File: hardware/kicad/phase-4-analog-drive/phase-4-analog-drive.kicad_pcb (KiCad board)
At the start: 2 copper layers, 170 x 120 mm, 4 parts, among them J1 MONITOR_DRIVE, J2 HOST_CTRL, U1 SN74LV4066APWR, U2 SN74LVC1G66DBVR

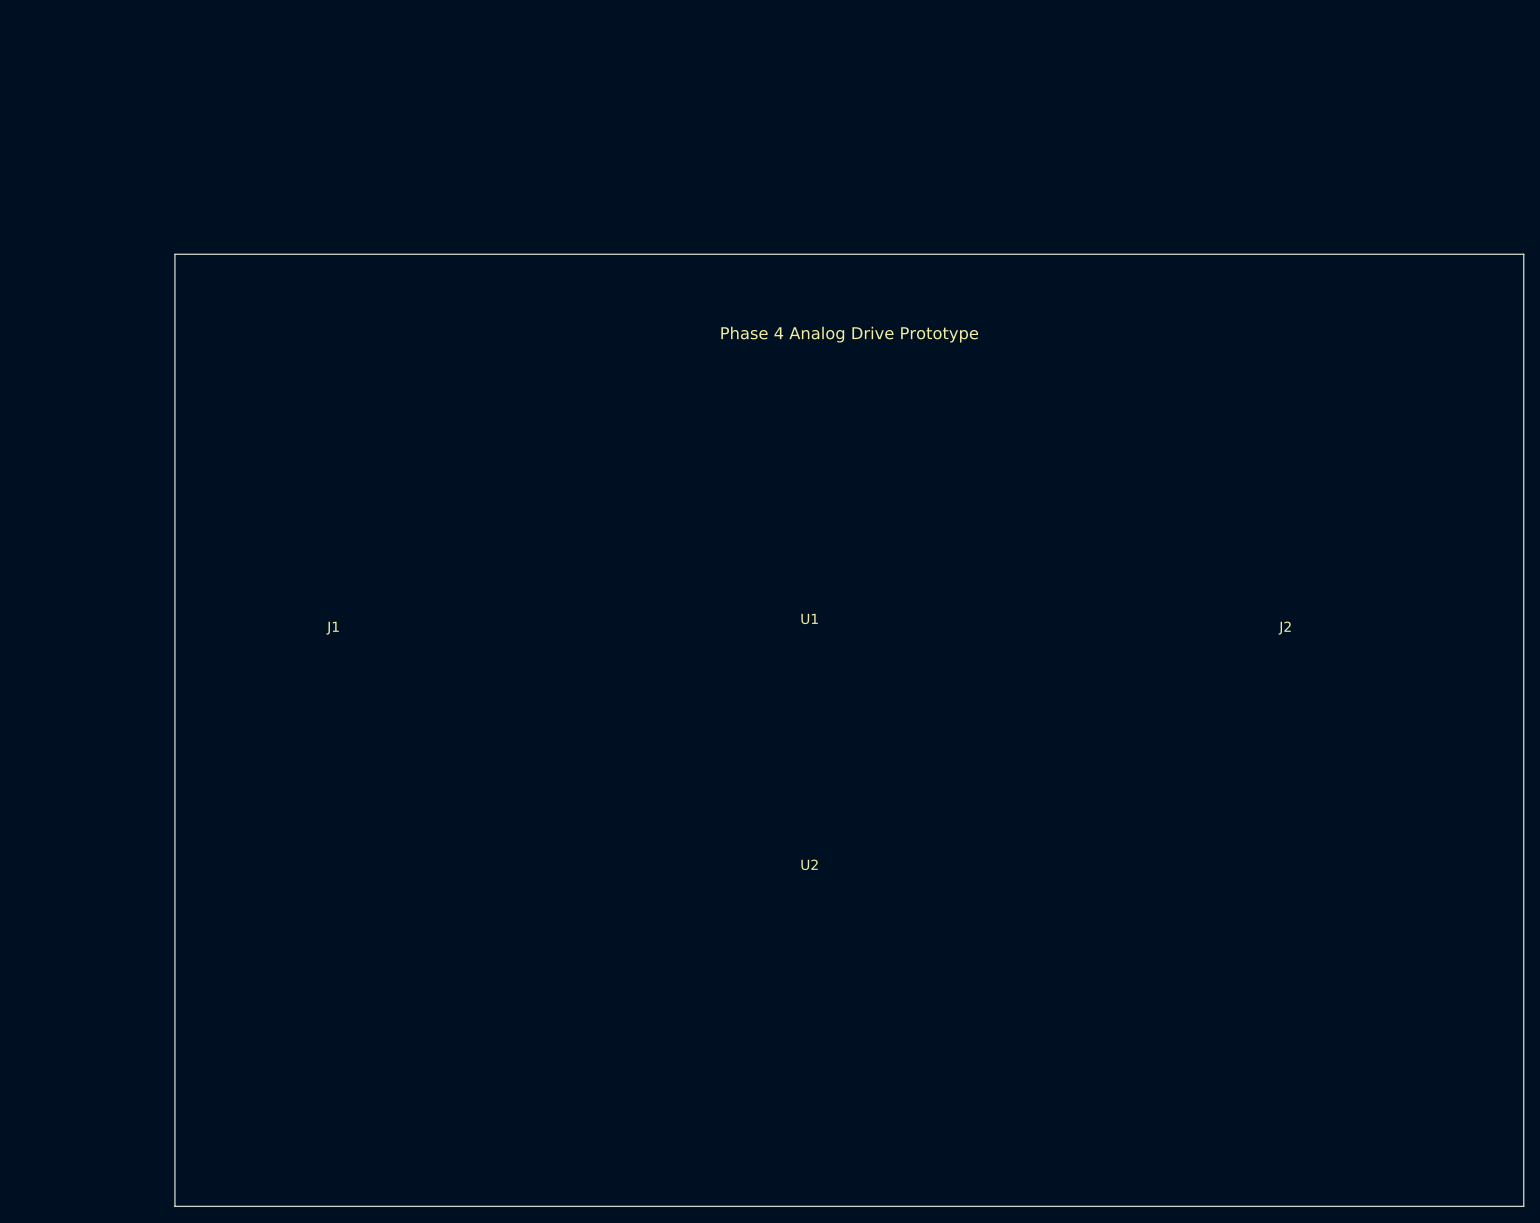
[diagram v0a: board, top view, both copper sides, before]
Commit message: Update phase 4 schema, WIP
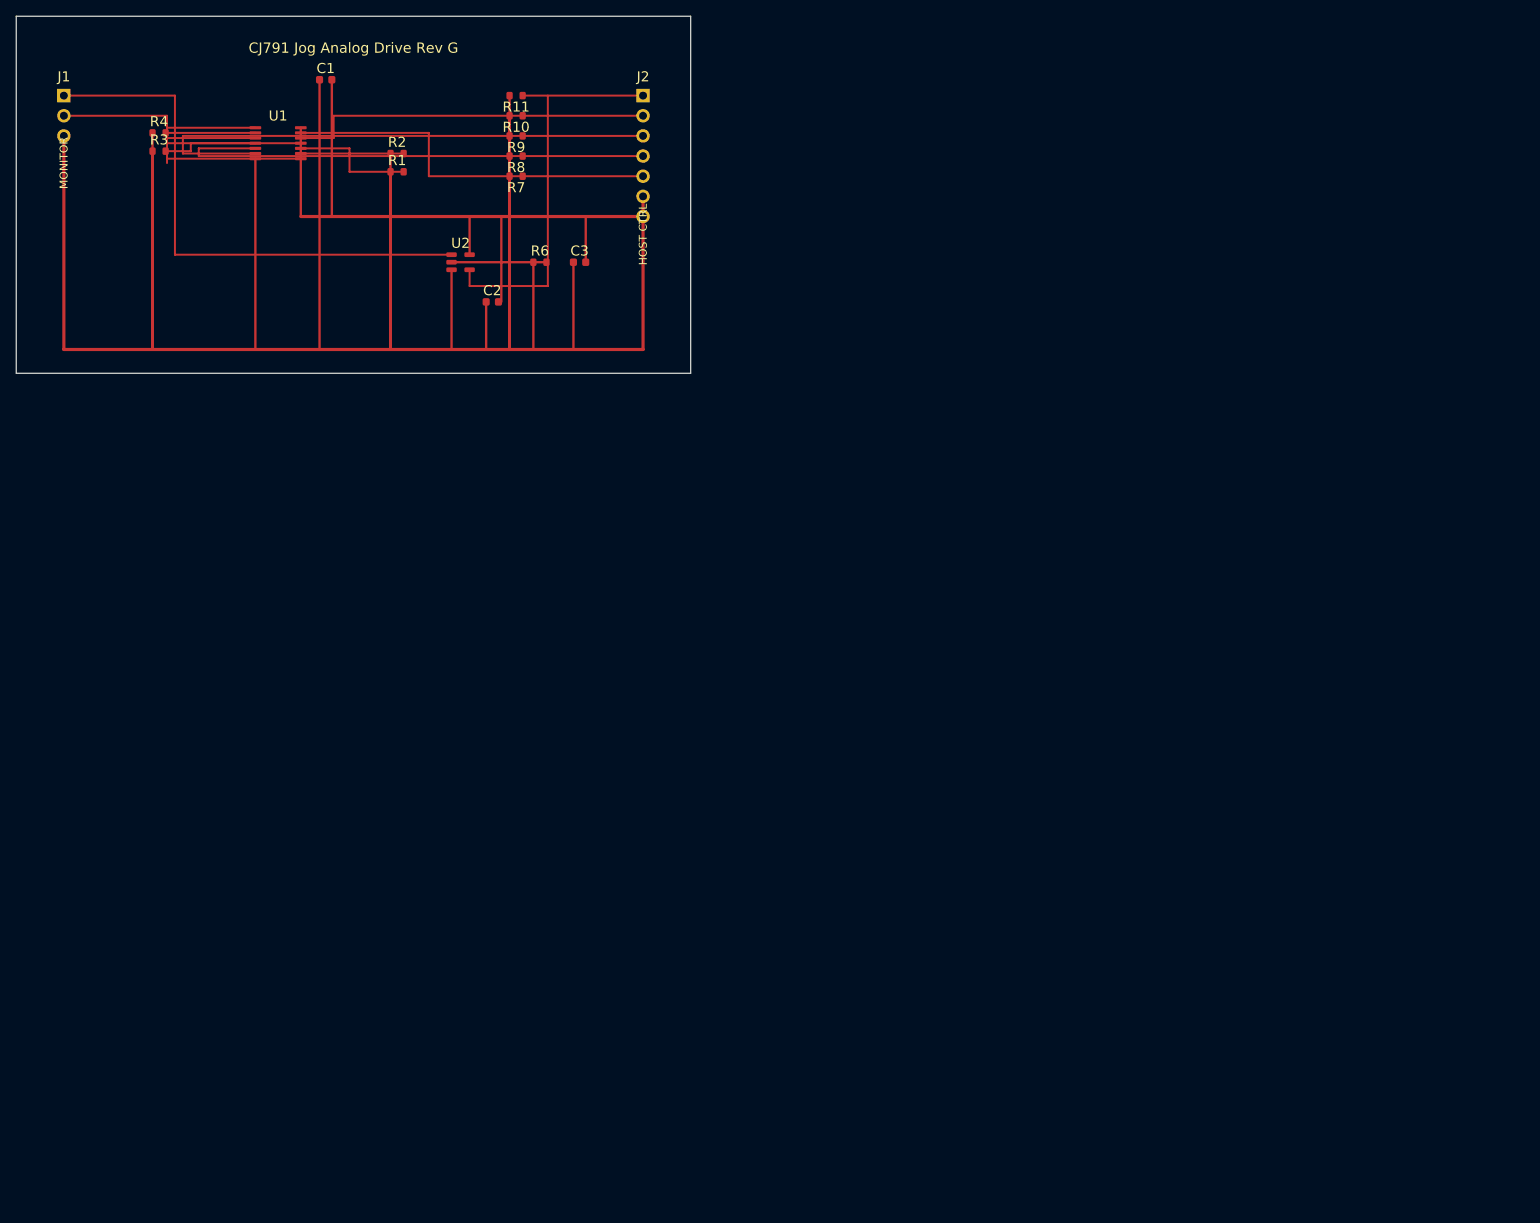
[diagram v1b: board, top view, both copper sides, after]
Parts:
- added C1: 100n, Capacitor_SMD:C_0603_1608Metric, F.Cu at (39.0, 8.00)
- added C2: 100n, Capacitor_SMD:C_0603_1608Metric, F.Cu at (60.0, 36.0)
- added C3: 1u, Capacitor_SMD:C_0603_1608Metric, F.Cu at (71.0, 31.0)
- added R1: 30k, Resistor_SMD:R_0603_1608Metric, F.Cu at (48.0, 19.6)
- added R10: 100k, Resistor_SMD:R_0603_1608Metric, F.Cu at (63.0, 12.5)
- added R11: 100k, Resistor_SMD:R_0603_1608Metric, F.Cu at (63.0, 10.0)
- added R2: 10k, Resistor_SMD:R_0603_1608Metric, F.Cu at (48.0, 17.3)
- added R3: 3.3k, Resistor_SMD:R_0603_1608Metric, F.Cu at (18.0, 17.0)
- added R4: 22k, Resistor_SMD:R_0603_1608Metric, F.Cu at (18.0, 14.7)
- added R6: 22k, Resistor_SMD:R_0603_1608Metric, F.Cu at (66.0, 31.0)
- added R7: 100k, Resistor_SMD:R_0603_1608Metric, F.Cu at (63.0, 20.2)
- added R8: 100k, Resistor_SMD:R_0603_1608Metric, F.Cu at (63.0, 17.6)
- added R9: 100k, Resistor_SMD:R_0603_1608Metric, F.Cu at (63.0, 15.1)
- U1: value SN74LV4066APWR -> MC74HC4066ADTR2G
- U2: value SN74LVC1G66DBVR -> 74LVC1G66LT05ARCQ
- moved J2 107.1 mm to (79.0, 10.0)
- moved U1 92.7 mm to (33.0, 16.0)
- moved U2 90.4 mm to (56.0, 31.0)
- moved J1 77.8 mm to (6.00, 10.0)
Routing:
- net /GND: track 0.00 -> 449.3 mm
- net /+3V3: track 0.00 -> 92.9 mm
- net /KEY_ADC2_BUS: track 0.00 -> 75.0 mm
- net /ADC2_DOWN_EN: track 0.00 -> 69.4 mm
- net /KEY_ADC1_BUS: track 0.00 -> 68.9 mm
- net /ADC2_RIGHT_EN: track 0.00 -> 64.1 mm
- net /ADC1_CENTER_EN: track 0.00 -> 51.1 mm
- net /ADC2_LEFT_EN: track 0.00 -> 48.6 mm
- net /ADC2_UP_EN: track 0.00 -> 45.9 mm
- net /ADC2_LEFT_SW: track 0.00 -> 15.9 mm
- net /ADC2_RIGHT_SW: track 0.00 -> 13.0 mm
- net /ADC2_DOWN_SW: track 0.00 -> 12.3 mm
- net /ADC1_CENTER_SW: track 0.00 -> 12.0 mm
- net /ADC2_UP_SW: track 0.00 -> 11.3 mm
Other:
- board size 170 x 120 mm -> 85 x 45 mm
- board text added: "CJ791 Jog Analog Drive Rev G"
- board text added: "HOST CTRL"
- board text added: "MONITOR"
- board text removed: "Phase 4 Analog Drive Prototype"
